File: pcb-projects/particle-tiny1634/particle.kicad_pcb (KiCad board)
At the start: 2 copper layers, 43.2 x 43.7 mm, 32 parts, among them CON1 AVR-ISP-6, IC1 ATTINY1634-SU, P1 TXN, P2 RXN, P3 TXS, P4 RXS, P5 TRXCH

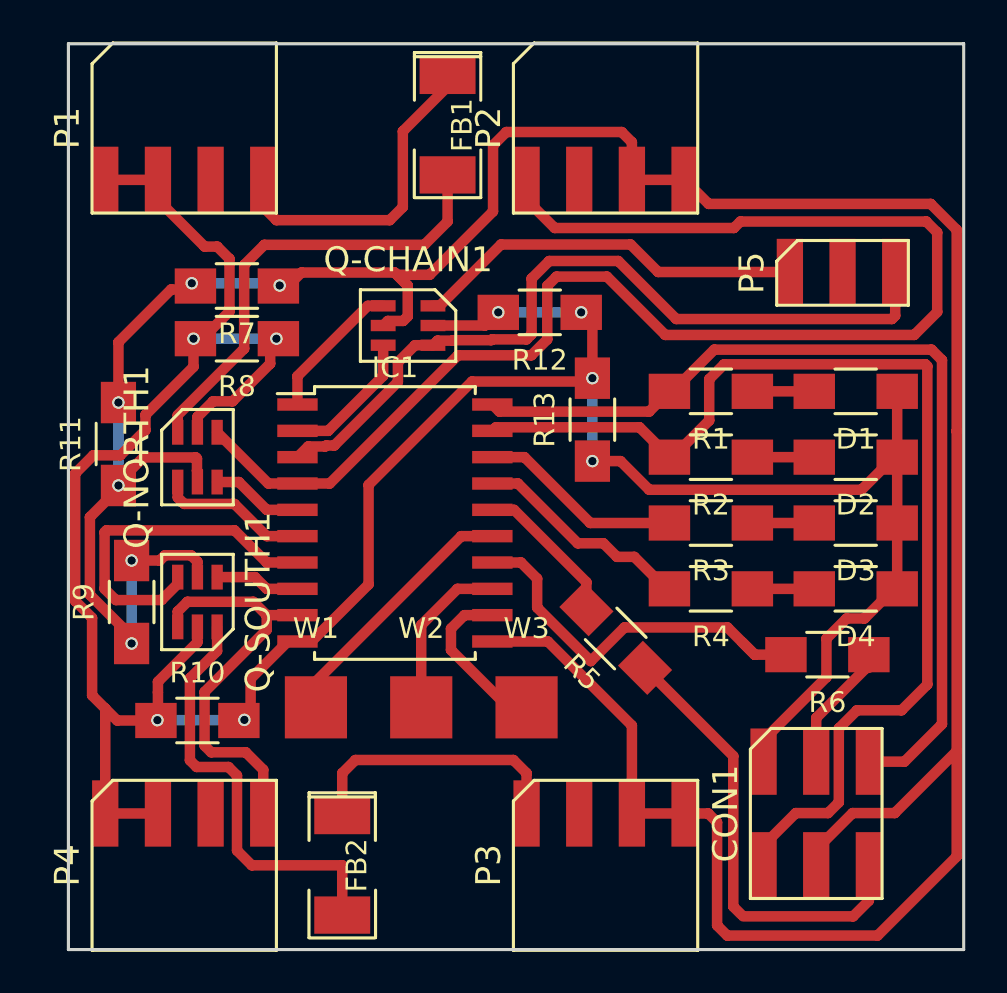
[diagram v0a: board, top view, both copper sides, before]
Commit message: cosmetics
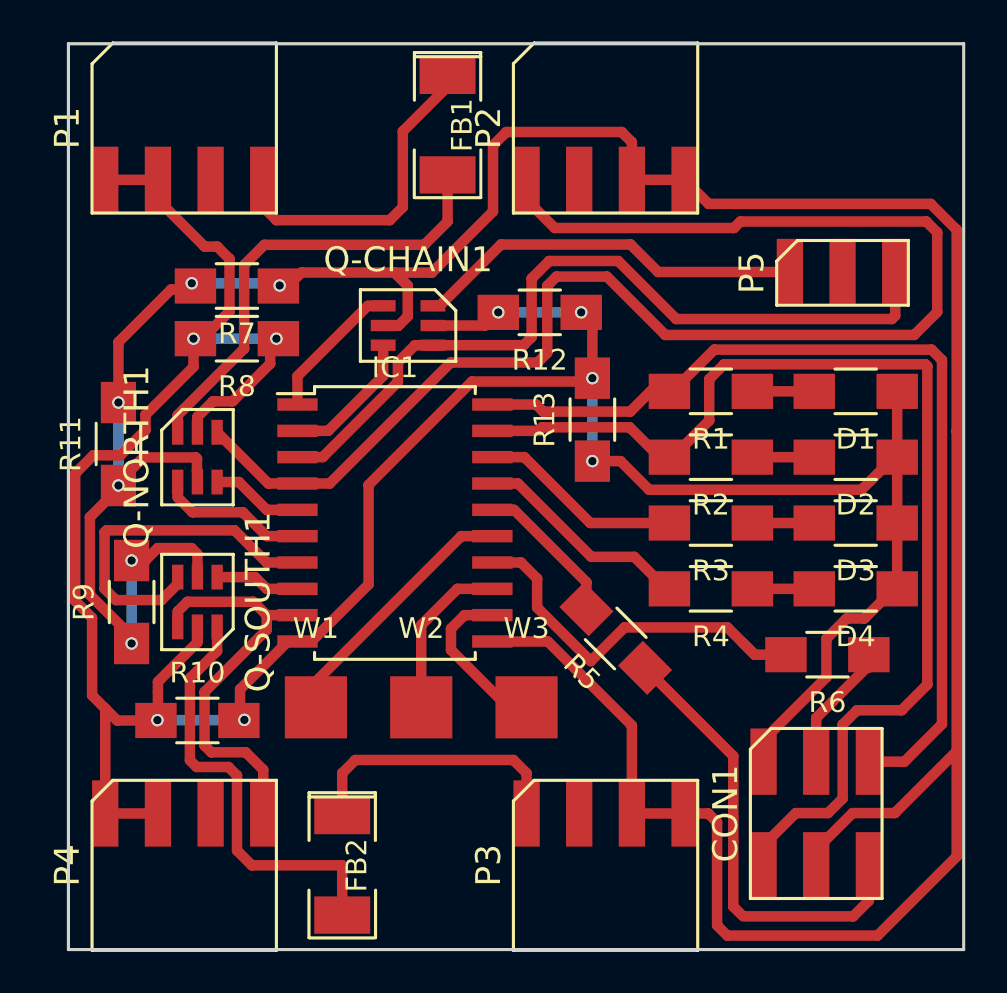
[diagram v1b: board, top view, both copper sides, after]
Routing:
- net VCC: track 159.3 -> 160.0 mm
